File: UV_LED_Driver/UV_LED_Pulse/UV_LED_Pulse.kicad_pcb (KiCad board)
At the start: 2 copper layers, 37.5 x 18.1 mm, 27 parts, among them J1 PWR/Signal, Q1 BC817, Q2 2N7002

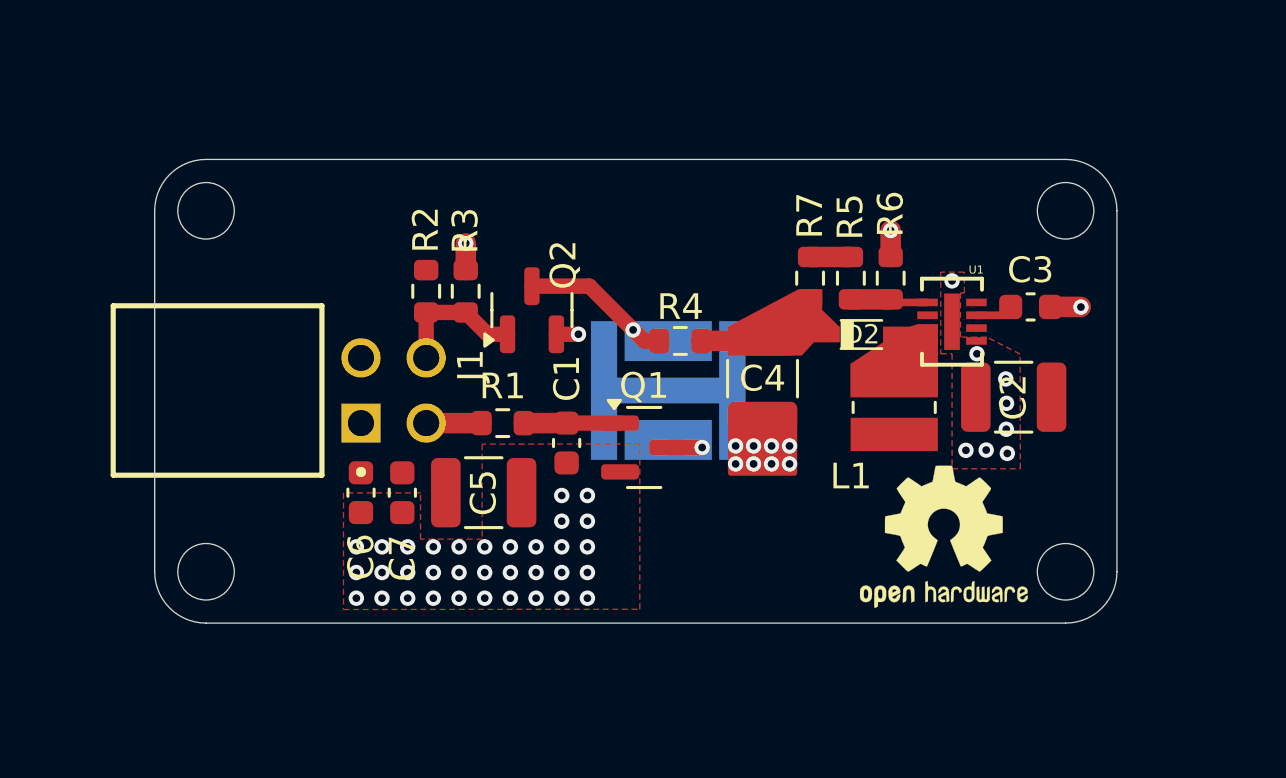
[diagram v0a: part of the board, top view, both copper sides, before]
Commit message: .
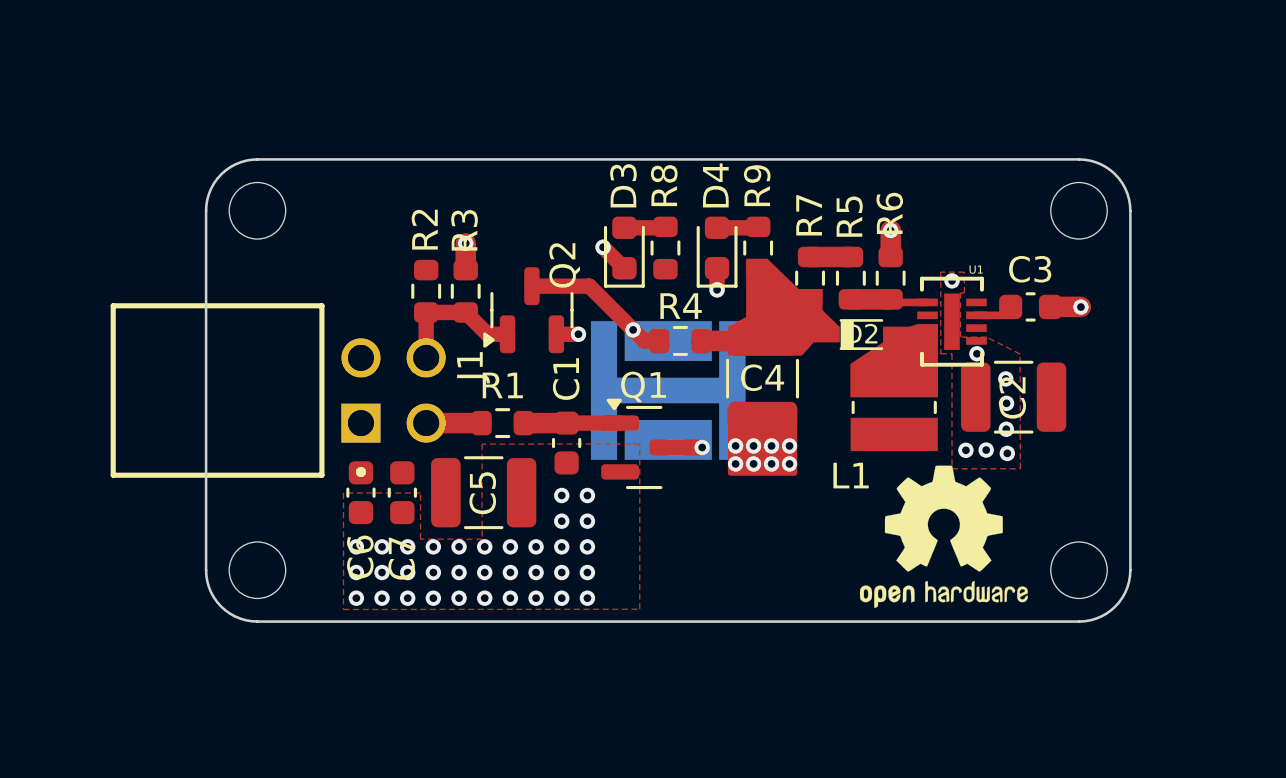
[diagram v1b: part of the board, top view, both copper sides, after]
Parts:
- removed the REF** at (69.6, 71.8)
- added D3: LED, LED_SMD:LED_0603_1608Metric, F.Cu at (84.9, 66.4)
- added D4: LED, LED_SMD:LED_0603_1608Metric, F.Cu at (88.5, 66.4)
- added R8: 600, Resistor_SMD:R_0603_1608Metric, F.Cu at (86.5, 66.4)
- added R9: 1k, Resistor_SMD:R_0603_1608Metric, F.Cu at (90.2, 66.4)
- moved REF** 2.00 mm to (70.6, 78.9)
- moved REF** 2.00 mm to (70.6, 64.9)
- moved REF** 0.53 mm to (102.6, 78.9)
- moved REF** 0.52 mm to (102.6, 64.9)
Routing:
- net GND: track 4.12 -> 6.13 mm, vias 54 -> 56
- net Net-(D4-A): track 0.00 -> 1.62 mm
- net Net-(D3-A): track 0.00 -> 1.62 mm
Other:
- board size 37.5 x 18.1 mm -> 36 x 18 mm
